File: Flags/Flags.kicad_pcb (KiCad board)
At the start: 2 copper layers, 63.5 x 41.9 mm, 22 parts, among them J1 Conn_01x07_Male, J2 Conn_01x06_Male, J3 Conn_01x03_Male, J4 Conn_01x04_Male, U1 74LS08, U2 74HC74, U3 74LS175

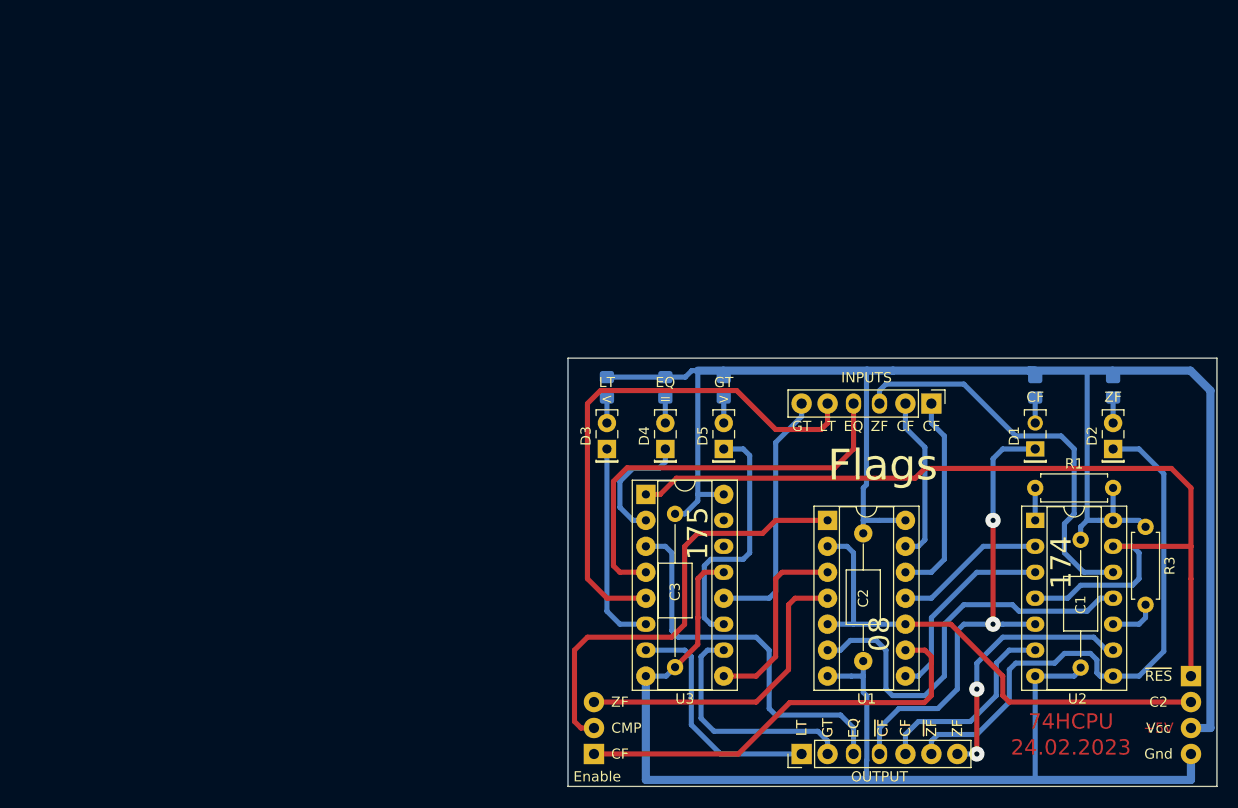
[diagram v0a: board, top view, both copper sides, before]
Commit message: Lost origin
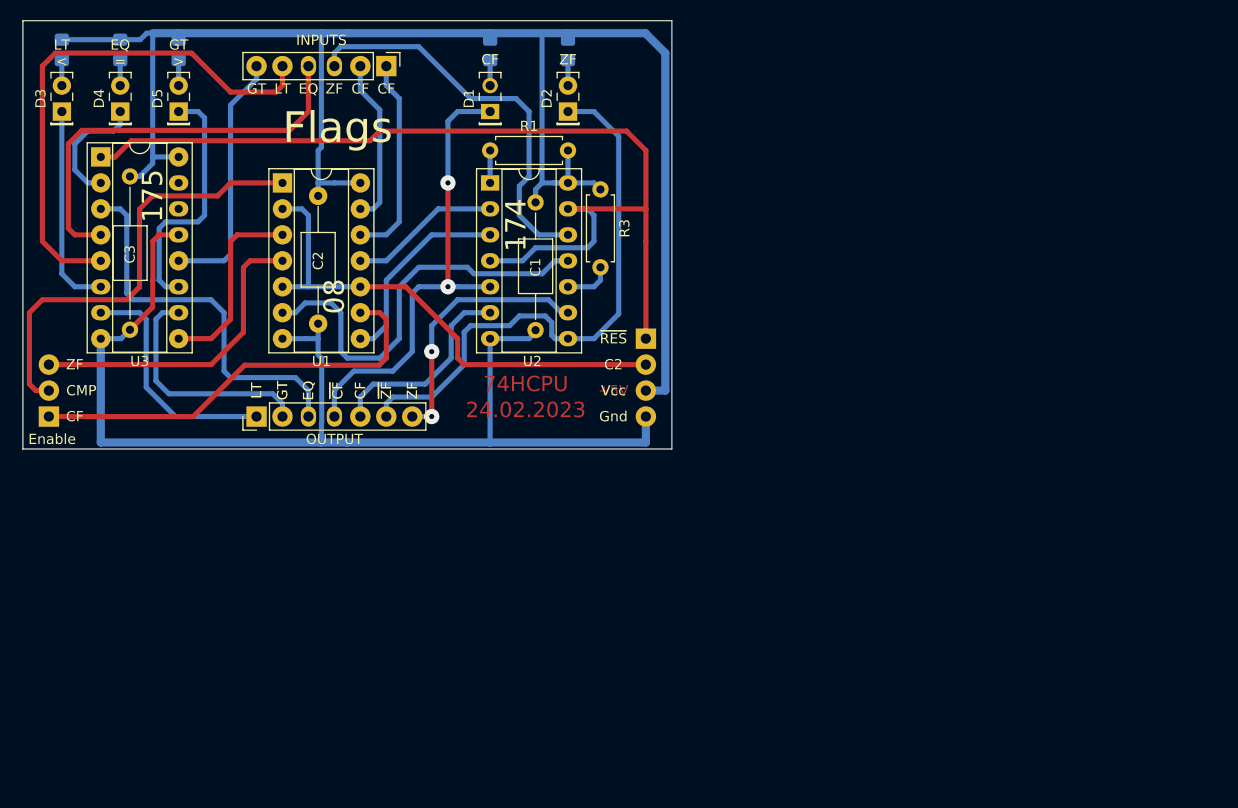
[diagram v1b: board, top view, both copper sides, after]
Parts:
- moved J4 62.7 mm to (78.7, 48.3)
- moved C3 62.7 mm to (28.3, 32.4)
- moved J3 62.7 mm to (20.3, 55.9)
- moved U1 62.7 mm to (43.2, 33.0)
- moved C1 62.7 mm to (67.9, 34.9)
- moved C2 62.7 mm to (46.7, 34.3)
- moved D1 62.7 mm to (63.5, 26.0)
- moved D3 62.7 mm to (21.6, 26.0)
- moved J1 62.7 mm to (40.6, 55.9)
- moved J2 62.7 mm to (53.3, 21.6)
- moved R1 62.7 mm to (63.5, 29.8)
- moved R2 62.7 mm to (63.5, 20.0)
- moved R3 62.7 mm to (74.3, 33.7)
- moved R5 62.7 mm to (21.6, 20.0)
- moved U2 62.7 mm to (63.5, 33.0)
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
